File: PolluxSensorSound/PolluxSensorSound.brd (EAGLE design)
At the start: 21.3 x 19 mm, 3 parts

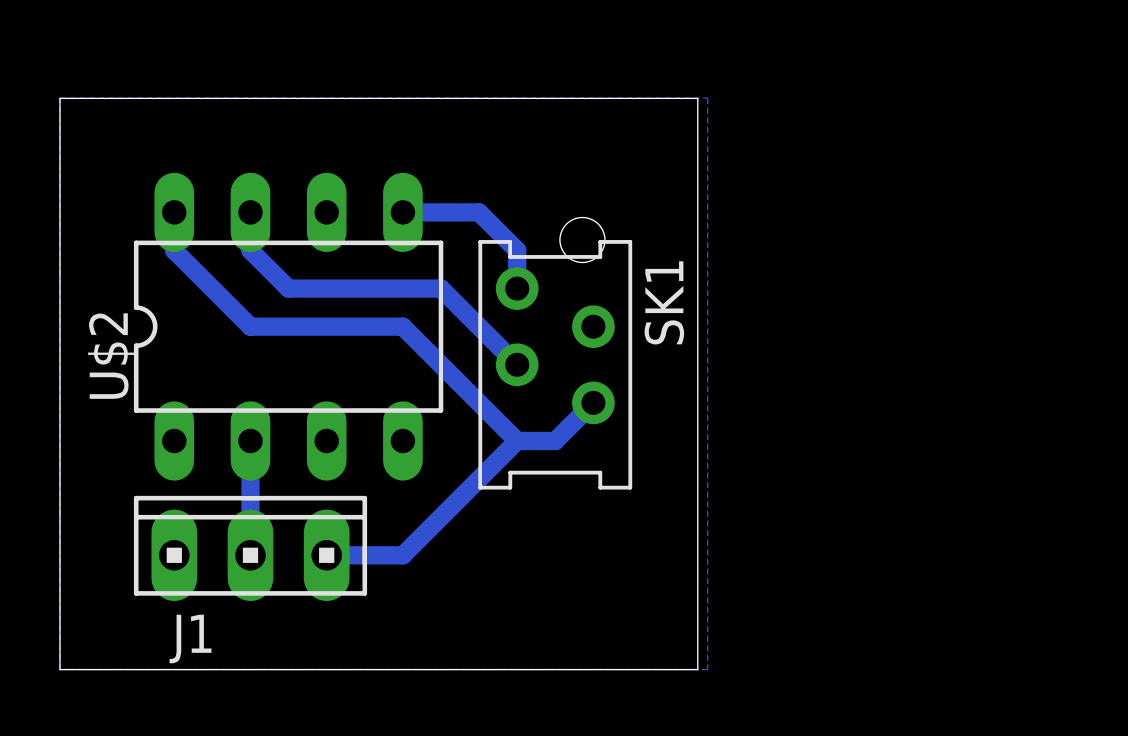
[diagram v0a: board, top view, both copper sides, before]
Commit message: improve sensor board
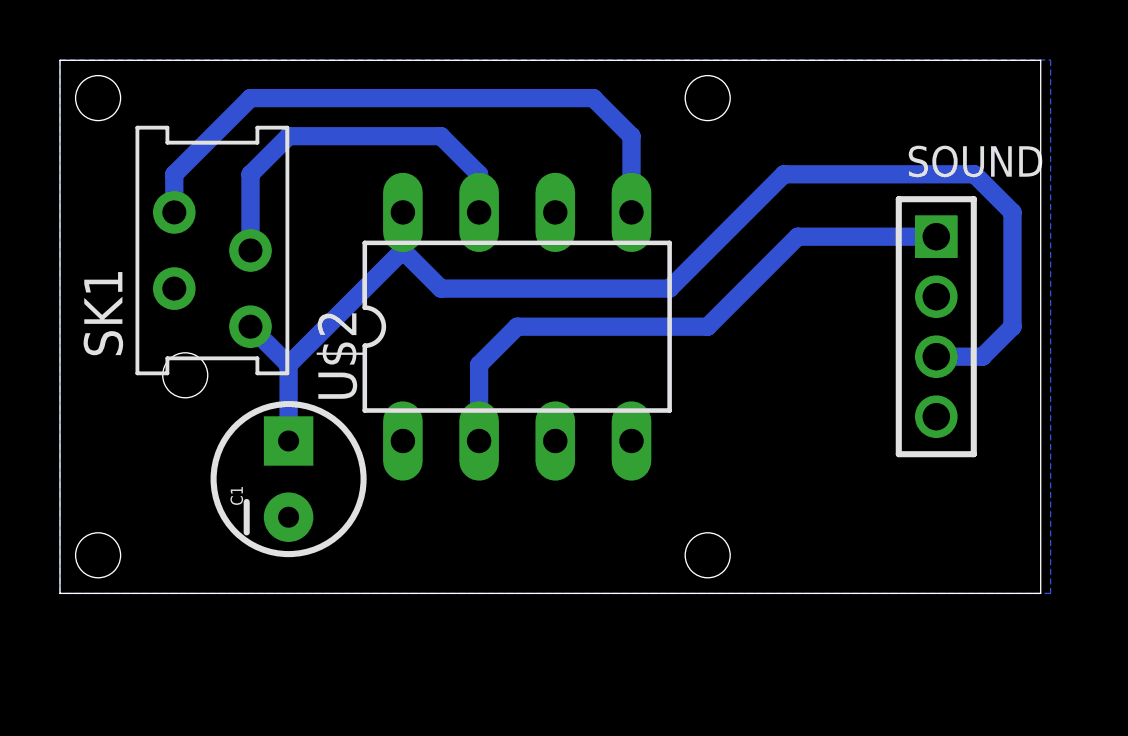
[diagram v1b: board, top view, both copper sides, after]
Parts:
- removed J1: (no value), con-amp:10X03MTA
- added C1: 1 uF, SparkFun:CPOL-RADIAL-10UF-25V
- added SOUND: (no value), pinhead-2:1X04M
- moved SK1 11.5 mm to (16.5, 16.5), turned to 90 degrees
- moved U$2 7.62 mm to (26.7, 16.5)
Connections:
- removed net N$2 (its old number): SK1.1, U$2.5
- new net SDA: SK1.4, U$2.5
- net 5V: now also C1.1, SK1.1, SOUND.3; no longer J1.1, SK1.4
- net GND: now also C1.2, SOUND.4; no longer J1.3
- net READ: now also SOUND.1; no longer J1.2
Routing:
- net SDA: track 0.00 -> 20.6 mm
- net READ: track 3.81 -> 19.5 mm
- net 5V: track 26.3 -> 40.7 mm
- net N$2 (its old number): track 5.61 -> 0.00 mm
- net N$2: track 11.7 -> 12.5 mm
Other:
- board size 21.3 x 19 mm -> 32.7 x 17.8 mm
